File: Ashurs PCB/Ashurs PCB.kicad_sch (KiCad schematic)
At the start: 0 parts

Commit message: PCB check by david push
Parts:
- added C1: 100nF, Capacitor_SMD:C_0603_1608Metric, symbol Device:C
- added C14: 120nF, Capacitor_SMD:C_0603_1608Metric, symbol Device:C
- added C2, C5, C6: 1uF, Capacitor_SMD:C_0603_1608Metric, symbol Device:C
- added C7: 4.7uF, Capacitor_SMD:C_0603_1608Metric, symbol Device:C
- added C8: 0.1uF, Capacitor_SMD:C_0603_1608Metric, symbol Device:C
- added D3: SP0503BAHTG, Package_TO_SOT_SMD:SOT-143, symbol USB Diode:SP0503BAHTG
- added D4: LED, Diode_SMD:D_0201_0603Metric, symbol Device:LED
- added H1, H2, H3, H4: MountingHole, MountingHole:MountingHole_2.2mm_M2, symbol Mechanical:MountingHole
- added J1: 3220-20-0200-00, footprint:322020020000, symbol 20 pin connector:3220-20-0200-00
- added J2: GSB1C41110SSHR, footprint:AMPHENOL_GSB1C41110SSHR, symbol USB-C:GSB1C41110SSHR
- added J3: 1984617, footprint:PHOENIX_1984617, symbol 2 pin v2:1984617
- added J4: 647676-2, footprint:TE_647676-2, symbol 647676-2:647676-2
- added LS1: AT-1438-TWT-R, footprint:XDCR_AT-1438-TWT-R, symbol AT-1438-TWT-R:AT-1438-TWT-R
- added Q1: NMOS, Package_TO_SOT_SMD:SOT-23, symbol Simulation_SPICE:NMOS
- added R1, R10, R11, R12, R15, R2, R8, R9: 10k, Resistor_SMD:R_0603_1608Metric, symbol Device:R
- added R13: 220, Resistor_SMD:R_0603_1608Metric, symbol Device:R
- added R14: R, Resistor_SMD:R_0603_1608Metric, symbol Device:R
- added R16, R17: 4.7K, Resistor_SMD:R_0603_1608Metric, symbol Device:R
- added R3, R4: 100k, Resistor_SMD:R_0603_1608Metric, symbol Device:R
- added R5: 22.1k, Resistor_SMD:R_0603_1608Metric, symbol Device:R
- added R6: 47.5k, Resistor_SMD:R_0603_1608Metric, symbol Device:R
- added R7: 5.1k, Resistor_SMD:R_0603_1608Metric, symbol Device:R
- added U1: BNO055, footprint:LGA28R50P4X10_380X520X100, symbol BNO055:BNO055
- added U3: SST25VF010A-33-4C-SAE, footprint:SOIC8_SA_SST_MCH, symbol Flash Storage:SST25VF010A-33-4C-SAE
- added U4: BMP390, footprint:10LGA_2X2X0p75_BOS, symbol Altimeter:BMP390
- added U5: CP2102N-A02-GQFN20, footprint:QFN20_CP2102N_SIL, symbol USB Interface:CP2102N-A02-GQFN20
- added U6: ${SIM.PARAMS}, Package_SO:SOIC-8-1EP_3.9x4.9mm_P1.27mm_EP2.29x3mm, symbol Simulation_SPICE:OPAMP
- added Y2: ECS-327TXO-33-TR, footprint:OSC_ECS-327TXO-33-TR, symbol Resonator Clock:ECS-327TXO-33-TR
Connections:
- new net: C2.1, U1.9 (CAP)
- new net: LS1.N, Q1.1 (D)
- new net: J2.A5 (CC1), J2.B5 (CC2), R7.1
- new net: J3.1, R9.1, U6.1 (+)
- new net: R11.2, R12.1, U6.2 (-)
- new net: D3.3, J2.A6 (DP1), J2.B6 (DP2), U5.4 (D+)
- new net: D3.4, J2.A7 (DN1), J2.B7 (DN2), U5.5 (D-)
- new net: R5.1, R6.2, U5.8 (VBUS)
- new net: R8.1, U5.13 (WAKEUP)
- new net: D4.1 (K), R13.1
- new net +3V3: C1.2, C14.1, C5.1, C6.1, C7.2, C8.2, J1.1, J1.2, LS1.P, R1.1, R10.1, R11.1, R14.1, R15.1, R16.2, R17.2, R2.1, R3.1, R4.1, R8.2, U1.28 (VDDIO), U1.3 (VDD), U3.8 (VDD), U4.1 (VDDIO), U4.10 (VDD), U4.5 (SDO), U4.6 (CSB), U5.6 (VDD), Y2.4 (SUPPLY_VOLTAGE)
- new net Altimeter_SCL: R17.1, U4.2 (SCK)
- new net Altimeter_SDA: R16.1, U4.4 (SDI)
- new net Buzzer: Q1.2 (G)
- new net COOLLED: D4.2 (A)
- new net Flash_CE: U3.1 (*CE)
- new net Flash_Hold: U3.7 (*HOLD)
- new net Flash_SCK: U3.6 (SCK)
- new net Flash_SI: U3.5 (SI)
- new net Flash_SO: U3.2 (SO)
- new net Flash_WP: U3.3 (*WP)
- new net GND: C1.1, C14.2, C2.2, C5.2, C6.2, C7.1, C8.1, D3.1, J1.10, J1.12, J1.14, J1.16, J1.18, J1.20, J1.3, J1.4, J1.5, J1.6, J1.8, J2.A1_B12 (GND_A), J2.B1_A12 (GND_B), J2.SH1 (SHIELD), J2.SH2 (SHIELD__1), J2.SH3 (SHIELD__2), J2.SH4 (SHIELD__3), J4.2, Q1.3 (S), R12.2, R13.2, R6.1, R7.2, R9.2, U1.18 (COM2), U1.2 (GND), U1.25 (GNDIO), U1.5 (PS1), U1.6 (PS0), U3.4 (VSS), U4.3 (VSS), U4.8 (VSS), U4.9 (VSS), U5.12 (GND), U5.21 (EPAD), U5.3 (GND), U6.4 (V-), Y2.2 (GND)
- new net IMU_BL_IND: U1.10 (PIN10)
- new net IMU_SCL: R2.2, U1.19 (COM1)
- new net IMU_SDA: R1.2, U1.20 (COM0)
- new net IMU_nBOOTLOADPIN: R15.2, U1.4 (NBOOT_LOAD_PIN)
- new net IMU_nRESET: R14.2, U1.11 (NRESET)
- new net LIPO_POWER: J4.1
- new net PROG_NRST: J1.15
- new net PROG_SWCLK: J1.9, R3.2
- new net PROG_SWDIO: J1.7, R4.2
- new net PROG_SWO: J1.13
- new net RCC_OSC_IN: Y2.3 (OUTPUT)
- new net RCC_OSC_OUT: Y2.1 (OE)
- new net SWITCH: R10.2, U6.5
- new net USB_RSTB: U5.9 (RSTB)
- new net USB_RXD: U5.17 (RXD)
- new net USB_TXD: U5.18 (TXD)
- new net VBUS: D3.2, J2.A4_B9 (VBUS_A), J2.B4_A9 (VBUS_B), R5.2, U5.7 (VREGIN)
- new net VIN: J3.2, U6.3 (V+)
- no-connect marks 0 -> 19
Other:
- added sheet MCU (INTROmcu.kicad_sch)
- note added: "Altimeter"
- note added: "Buzzer"
- note added: "Cool LED"
- note added: "Data Switch"
- note added: "Flash"
- note added: "IMU"
- note added: "LIPO Terminal"
- note added: "Oscillator"
- note added: "Programmer"
- note added: "USB C Interface"

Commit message: post-david suggestions
u6 footprint, zener diode footprints, jumper footprints
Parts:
- U6: footprint Package_SO:SOIC-8-1EP_3.9x4.9mm_P1.27mm_EP2.29x3mm -> Package_TO_SOT_SMD:SOT-23-5
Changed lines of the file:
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@@
 			)
 		)
-		(property "Footprint" "Package_SO:SOIC-8-1EP_3.9x4.9mm_P1.27mm_EP2.29x3mm"
+		(property "Footprint" "Package_TO_SOT_SMD:SOT-23-5"
 			(at 68.58 158.75 0)
 			(effects

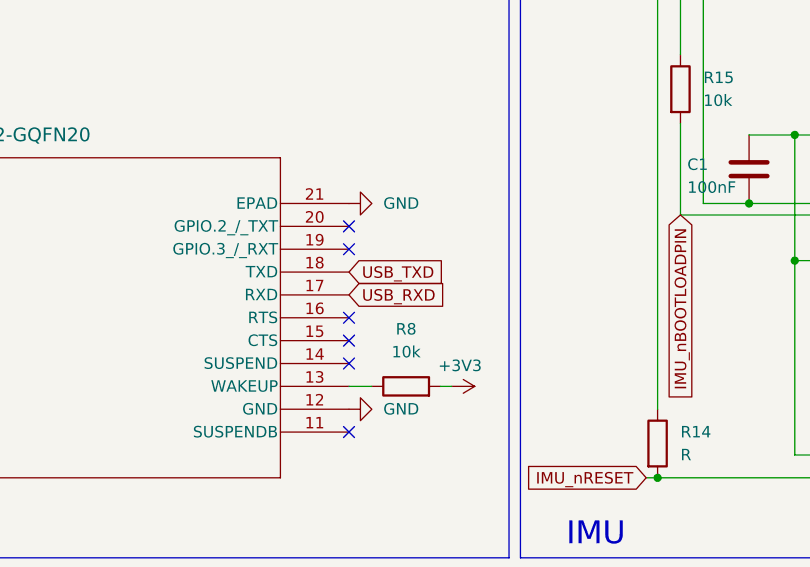
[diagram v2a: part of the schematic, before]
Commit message: Gerber and CSV's
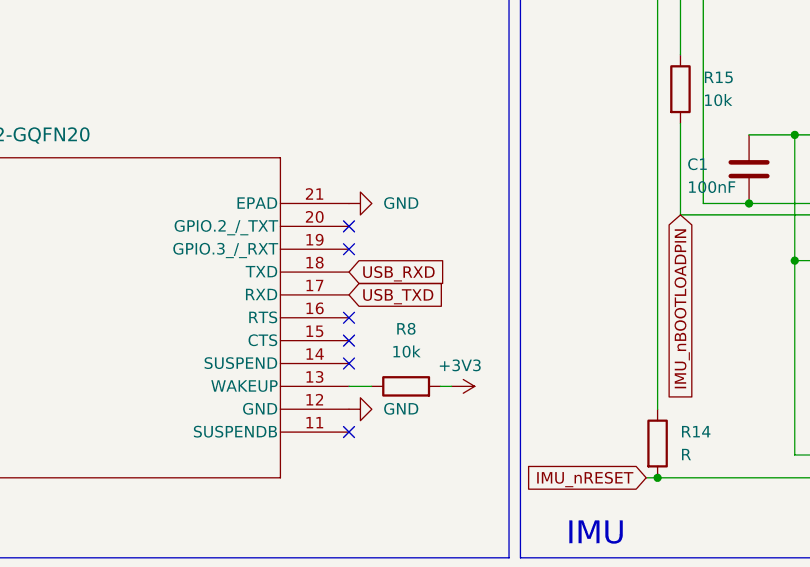
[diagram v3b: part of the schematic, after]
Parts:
- Q1: footprint Package_TO_SOT_SMD:SOT-23 -> Package_TO_SOT_SMD:TSOT-23
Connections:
- net USB_RXD: now also U5.18 (TXD); no longer U5.17 (RXD)
- net USB_TXD: now also U5.17 (RXD); no longer U5.18 (TXD)
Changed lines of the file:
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@@
 		)
 	)
-	(global_label "USB_TXD"
+	(global_label "USB_RXD"
 		(shape input)
 		(at 166.37 57.15 0)
@@
 		)
 		(property "Intersheetrefs" "${INTERSHEET_REFS}"
-			(at 177.5799 57.15 0)
+			(at 177.8823 57.15 0)
 			(effects
 				(font
@@
 		)
 	)
-	(global_label "USB_RXD"
+	(global_label "USB_TXD"
 		(shape input)
 		(at 166.37 59.69 0)
@@
 		)
 		(property "Intersheetrefs" "${INTERSHEET_REFS}"
-			(at 177.8823 59.69 0)
+			(at 177.5799 59.69 0)
 			(effects
 				(font
@@
 			)
 		)
-		(property "Footprint" "Package_TO_SOT_SMD:SOT-23"
+		(property "Footprint" "Package_TO_SOT_SMD:TSOT-23"
 			(at 96.52 121.92 0)
 			(effects
